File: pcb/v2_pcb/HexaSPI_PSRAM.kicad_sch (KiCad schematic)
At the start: 6 parts, among them U3 APS512XXN-OB9-BG

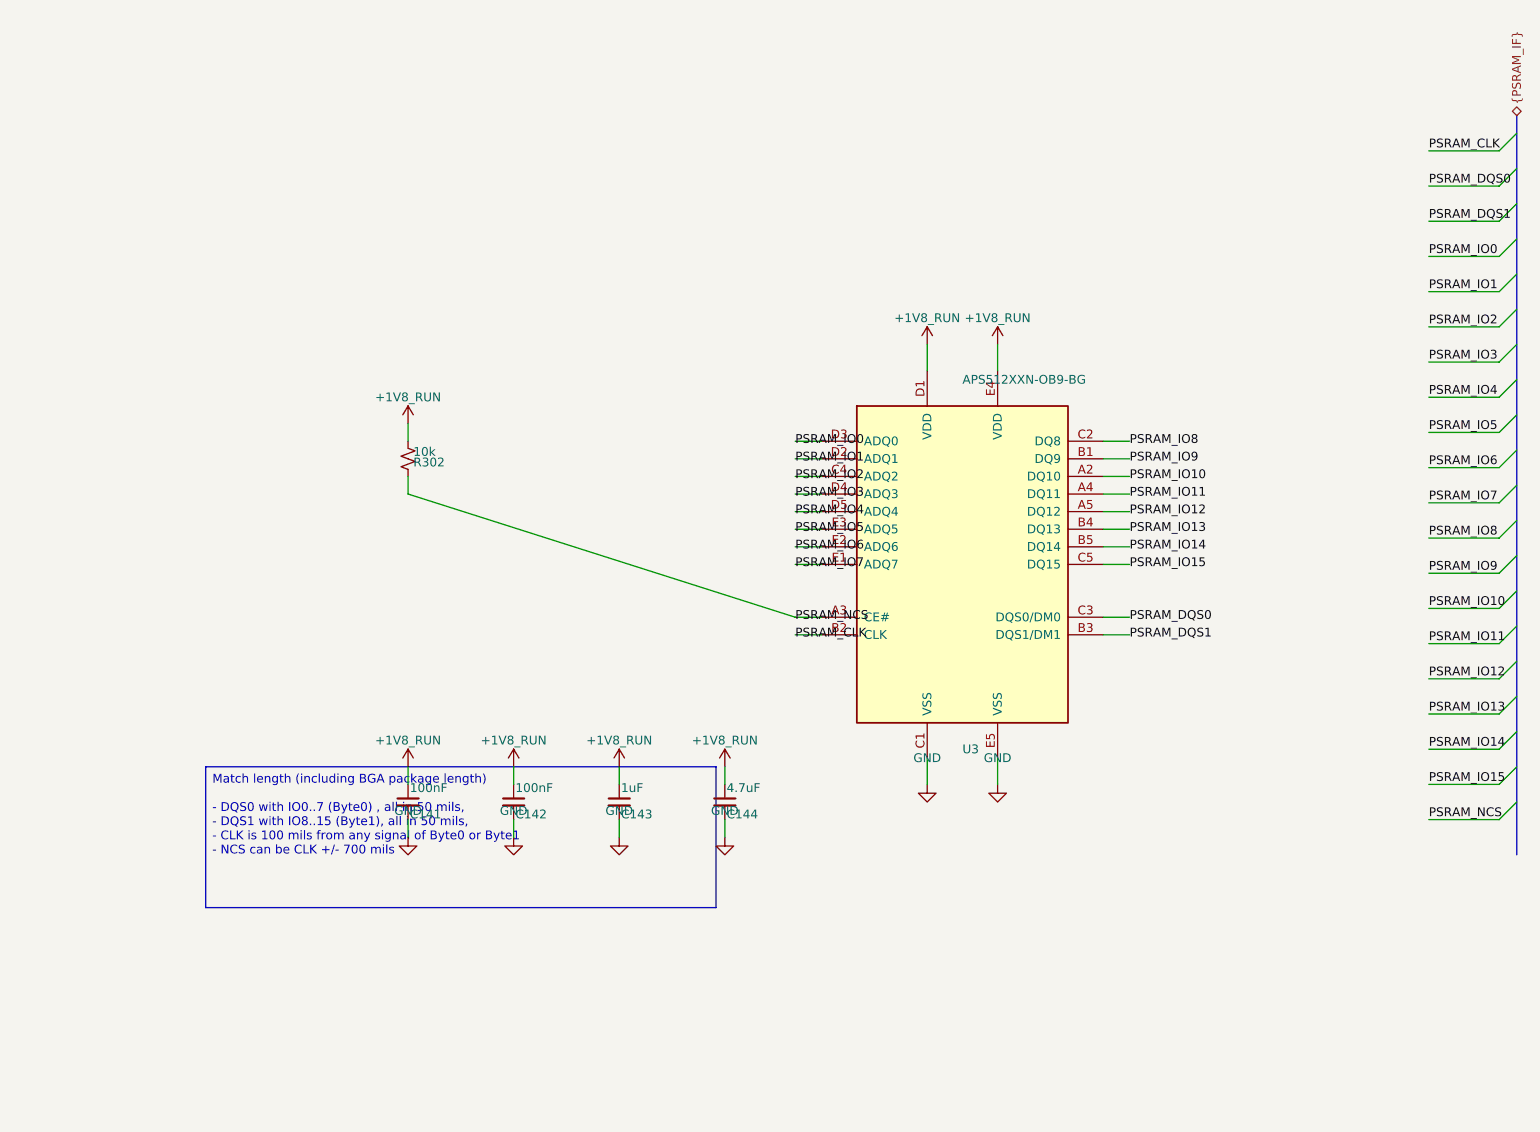
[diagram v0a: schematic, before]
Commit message: minor fixes
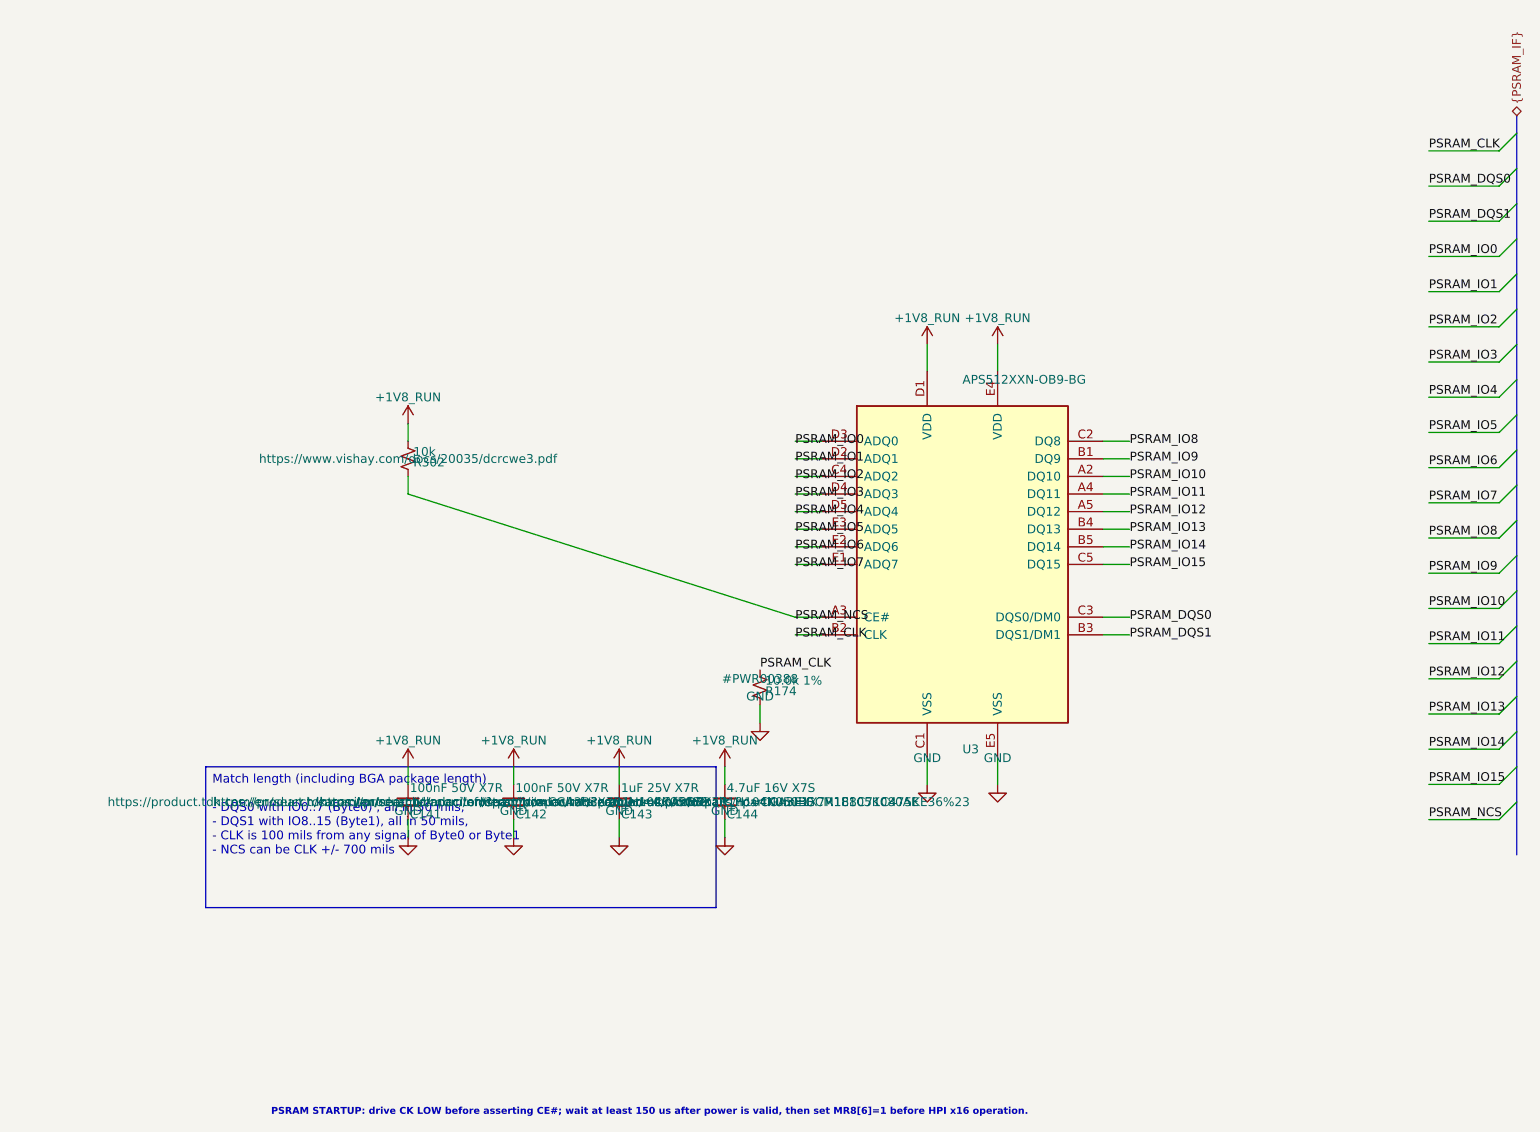
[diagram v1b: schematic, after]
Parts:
- added R174: 10.0k 1%, Resistor_SMD:R_0402_1005Metric, symbol Device:R_Small_US
- C141, C142: value 100nF -> 100nF 50V X7R; Dielectric (none) -> X7R; MPN (none) -> CGA2B3X7R1H104K050BE; Manufacturer (none) -> TDK; Qualification (none) -> AEC-Q200; Termination (none) -> Soft termination; Tolerance (none) -> ±10%; Voltage (none) -> 50 VDC
- C143: value 1uF -> 1uF 25V X7R; Dielectric (none) -> X7R; MPN (none) -> CGA3E1X7R1E105K080AE; Manufacturer (none) -> TDK; Qualification (none) -> AEC-Q200; Termination (none) -> Soft termination; Tolerance (none) -> ±10%; Voltage (none) -> 25 VDC
- C144: value 4.7uF -> 4.7uF 16V X7S; Dielectric (none) -> X7S; MPN (none) -> GCM188C71C475KE36D; Manufacturer (none) -> Murata; Qualification (none) -> AEC-Q200 powertrain/safety; Tolerance (none) -> ±10%; Voltage (none) -> 16 VDC
- R302: MPN (none) -> CRCW040210K0FKED; Manufacturer (none) -> Vishay; Power (none) -> 0.063 W; TCR (none) -> ±100 ppm/K; Tolerance (none) -> ±1%
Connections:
- net GND: now also R174.2
- net PSRAM_CLK: now also R174.1
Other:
- note added: "PSRAM STARTUP: drive CK LOW before asserting CE#; wait at least 150 us after power is valid, then set MR8[6]=1 before HPI x16 operation."

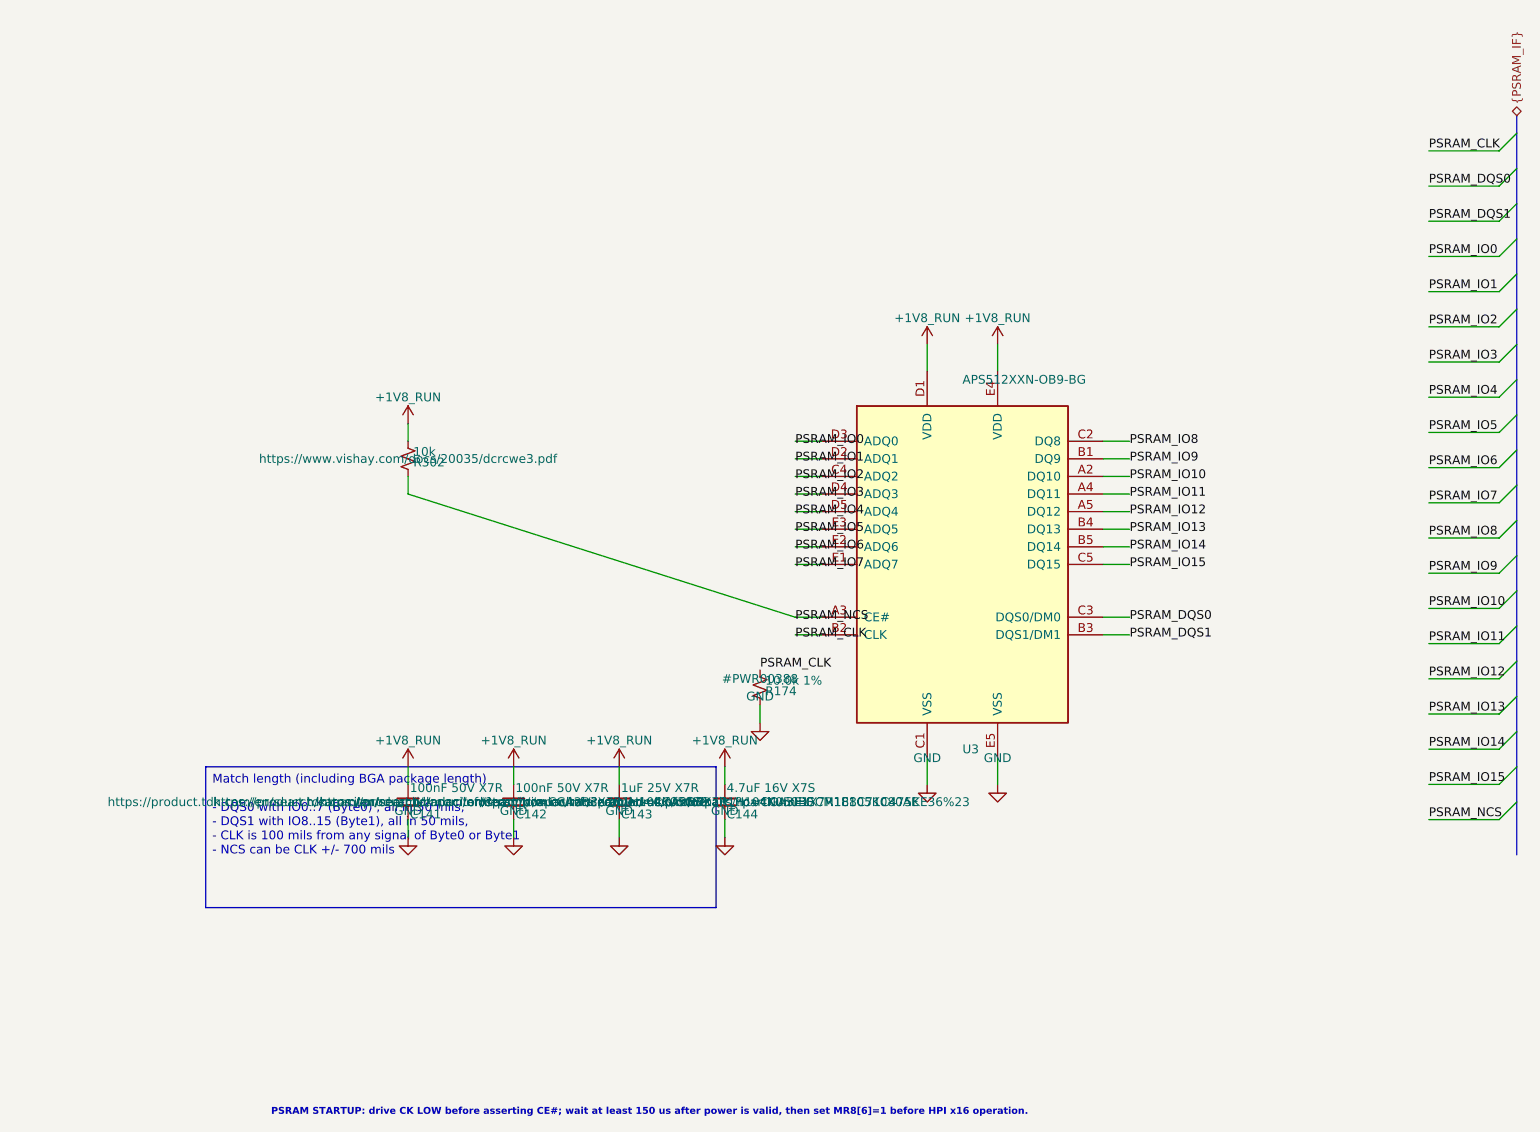
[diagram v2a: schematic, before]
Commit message: finish ram fanout
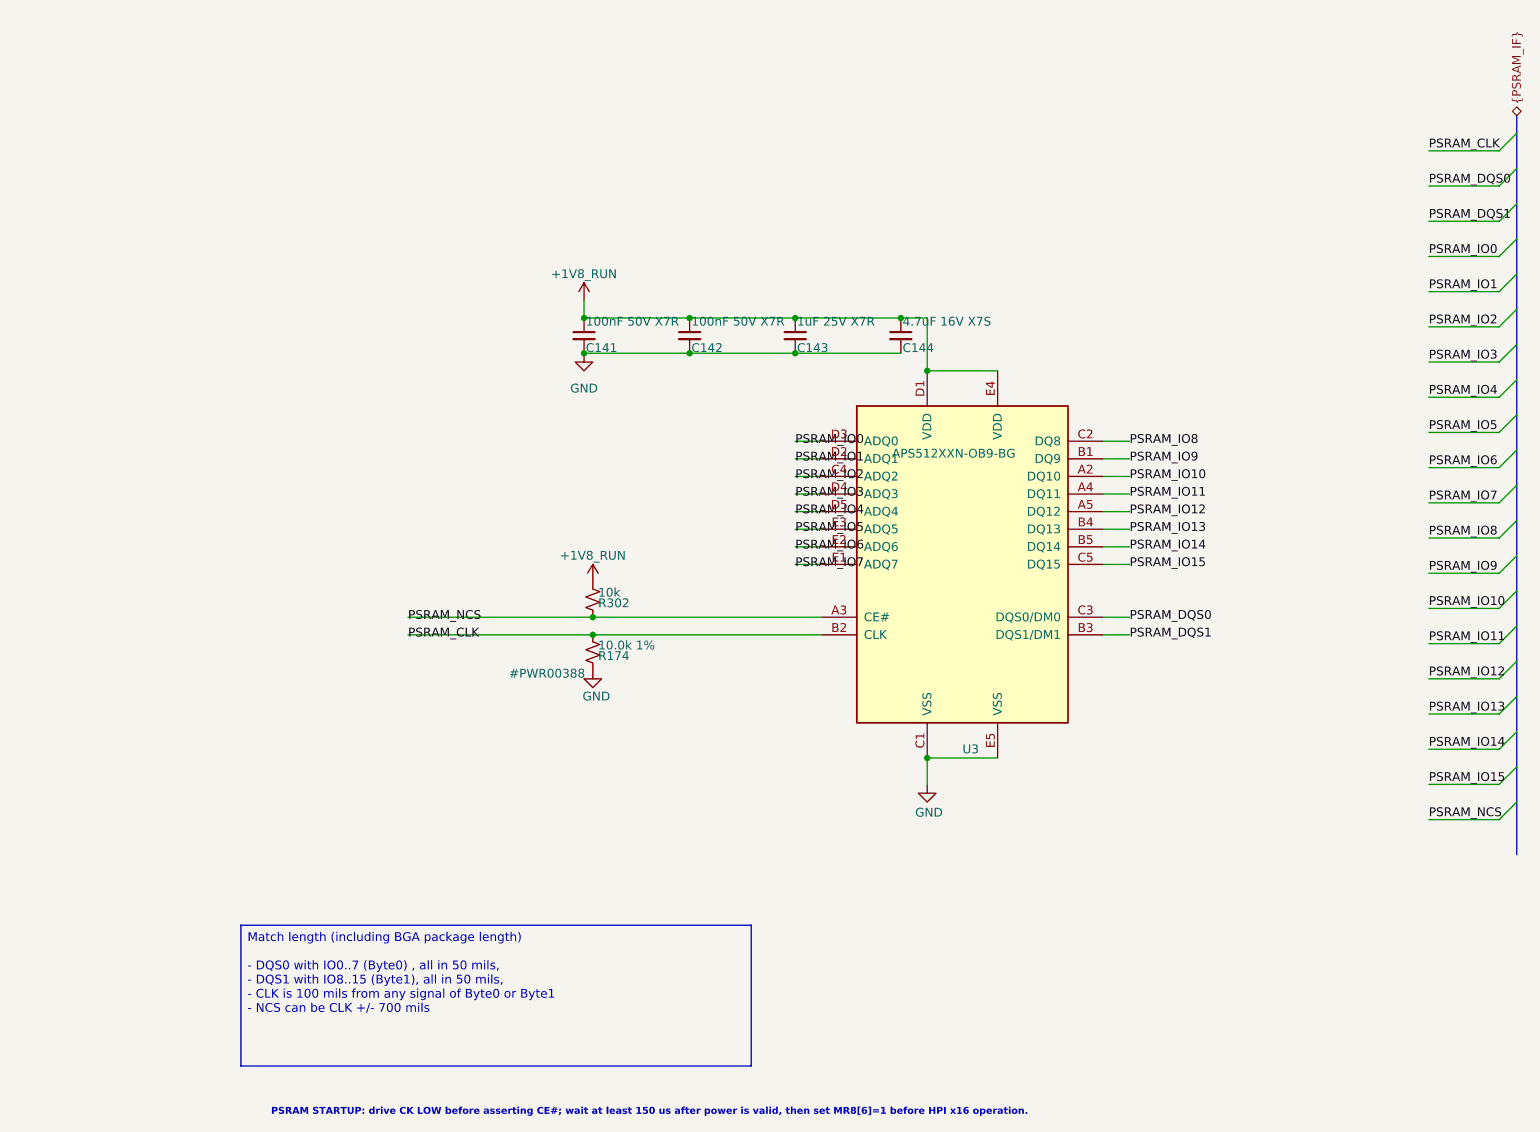
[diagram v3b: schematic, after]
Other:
- moved on the sheet: C141, C142, C143, C144
